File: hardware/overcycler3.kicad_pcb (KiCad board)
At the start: 2 copper layers, 200.7 x 99.1 mm, 309 parts, among them IC1 LM13700, IC2 LM13700, IC3 LM13700, J1 USB_B, J2 AudioJack3_Switch, J3 DIN-5_180degree, J4 AudioJack3_Switch, J5 AudioJack3_Switch, P1 FT232, P2 PANEL, Q1 2SC945, SW1 RESET, SW2 POWER, U1 XT26G02ELGIGA, U10 MCP4922-ESL, U11 SSI2144, U12 MCP4922-ESL, U13 SSI2144, U14 MCP4922-ESL, U15 SSI2144, U16 MCP4922-ESL, U17 SSI2144, U18 MCP4922-ESL, U19 SSI2144, U2 TL074, U20 AD5328B, U3 LPC1778FBD144, U4 TLV1543, U5 74HC138, U6 TL074, U7 AD5328B, U8 MCP4922-ESL, U9 SSI2144, Y1 12MHz

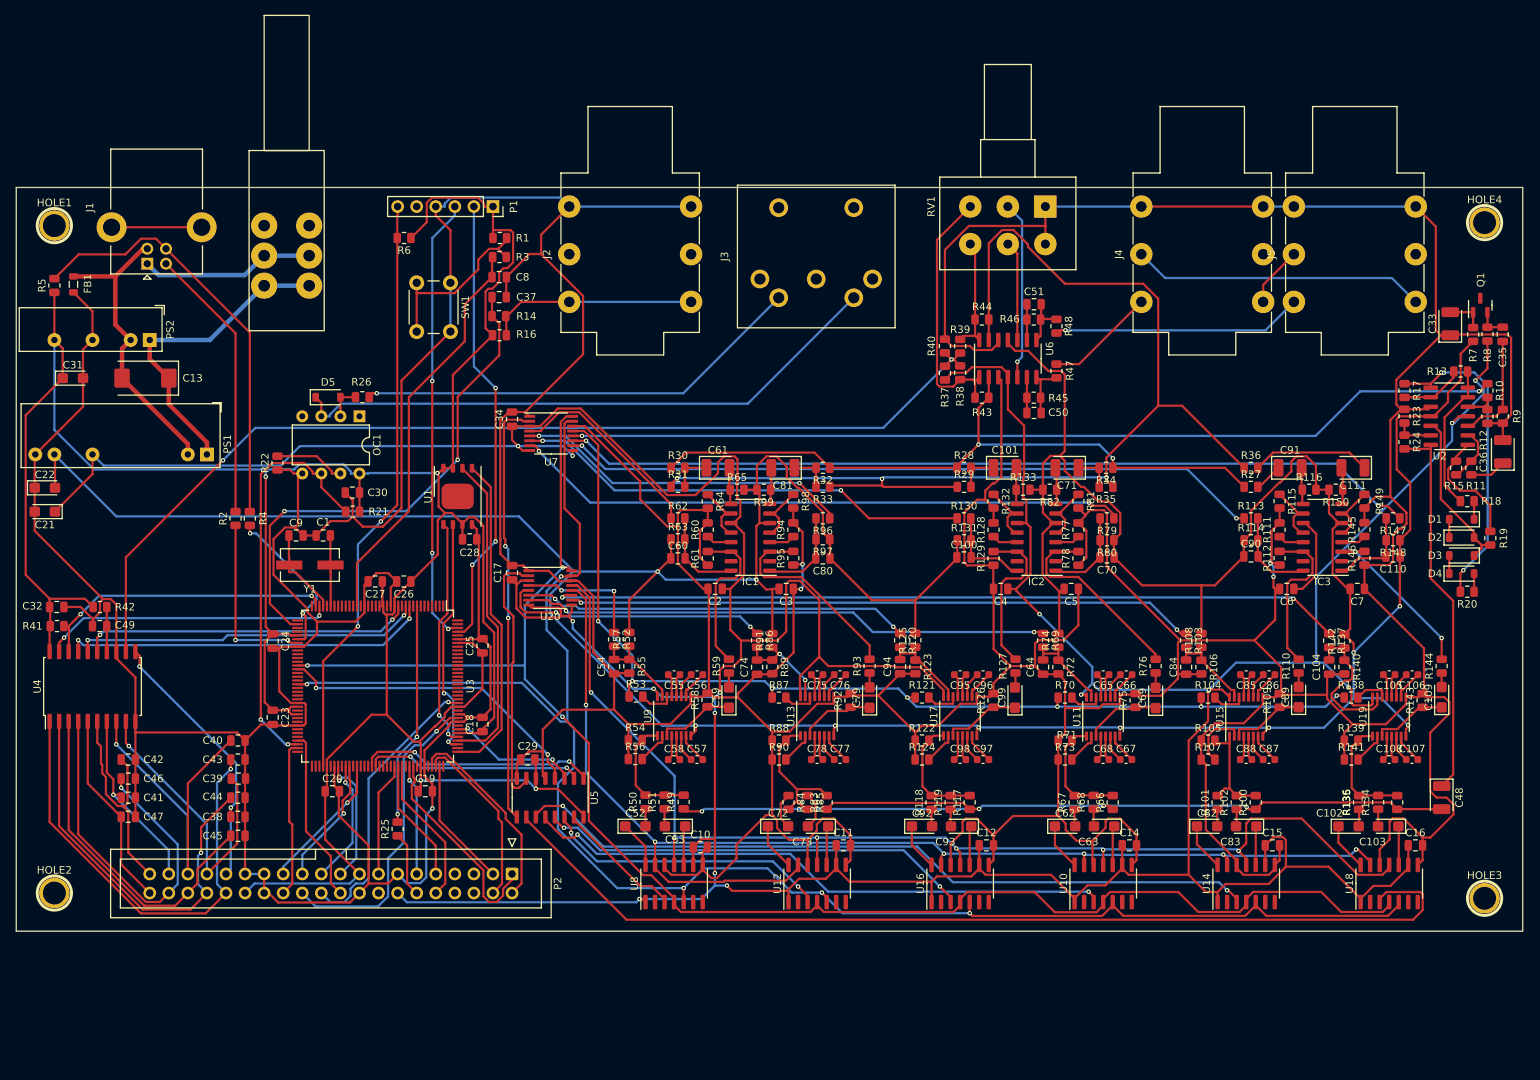
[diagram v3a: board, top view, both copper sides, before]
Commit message: hardware: improved draft routing
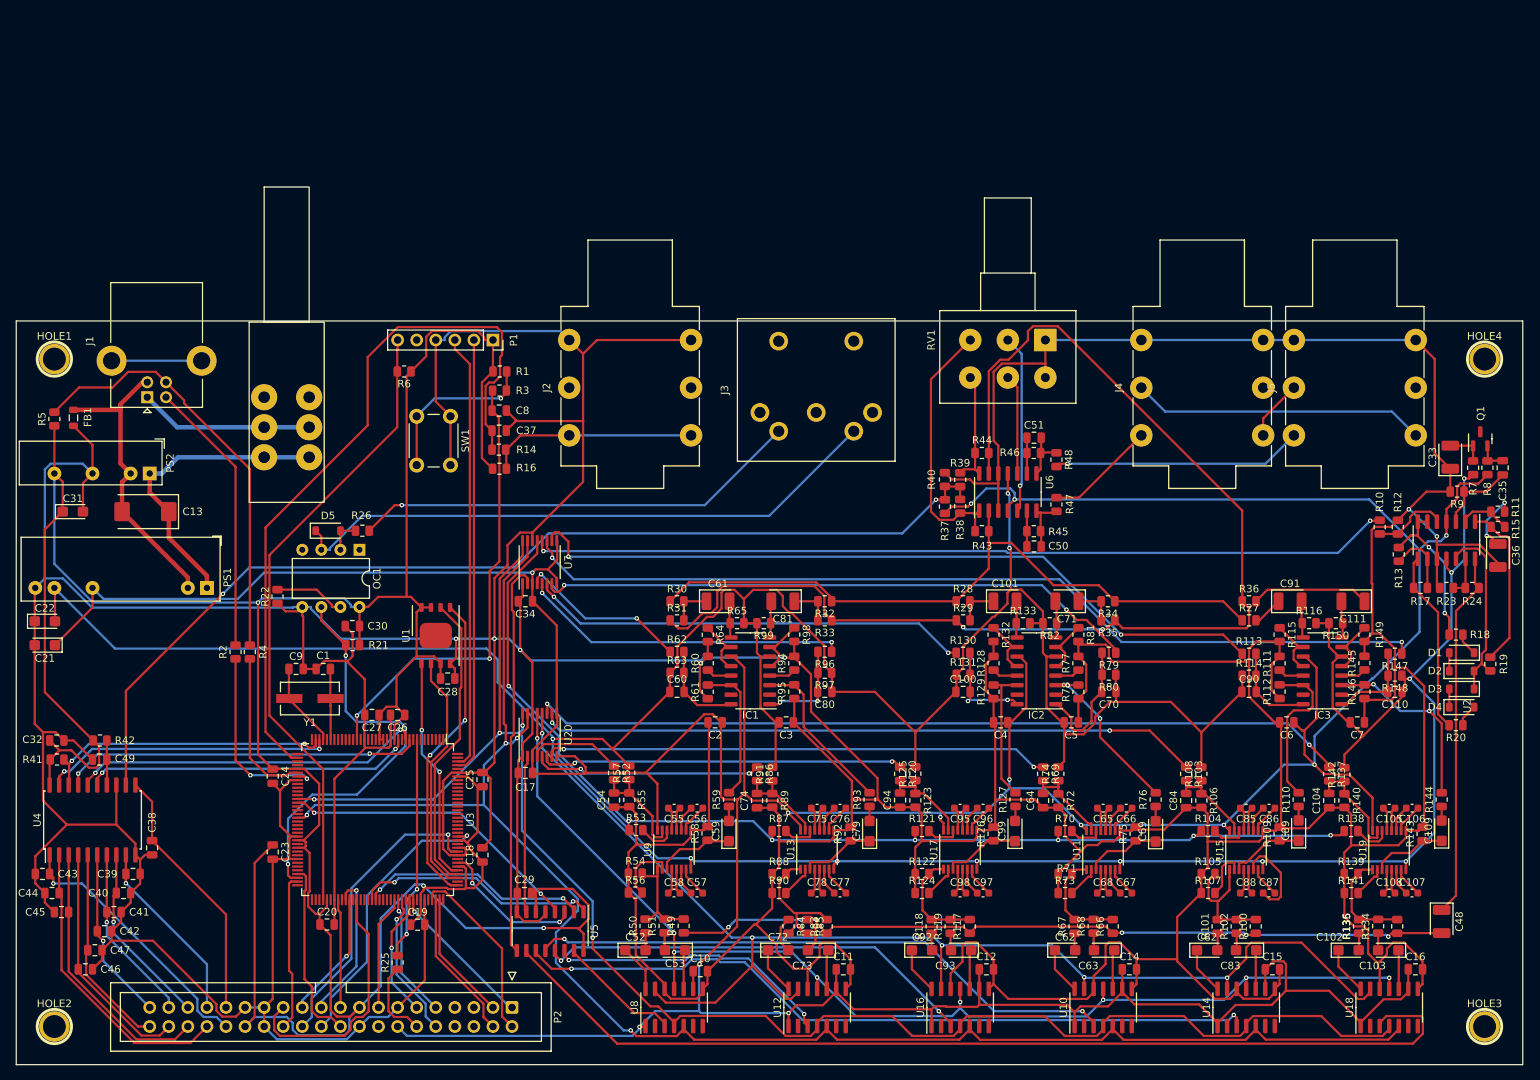
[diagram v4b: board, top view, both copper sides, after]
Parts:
- moved C43 30.2 mm to (23.8, 111.8), turned to 180 degrees
- moved C44 27.8 mm to (25.1, 114.3), turned to 180 degrees
- moved C17 26.7 mm to (88.1, 98.3), turned to 180 degrees
- moved R17 26.4 mm to (207.4, 73.7), turned to 0 degrees
- moved C46 26.0 mm to (29.5, 124.5)
- moved R13 25.7 mm to (204.5, 69.2), turned to -90 degrees
- moved C45 25.6 mm to (26.4, 116.8), turned to 180 degrees
- moved C40 25.4 mm to (34.6, 114.3)
- moved C34 24.3 mm to (88.1, 75.4), turned to 180 degrees
- moved R23 23.6 mm to (210.8, 73.7), turned to 0 degrees
- moved R10 23.2 mm to (201.9, 65.6)
- moved C42 23.1 mm to (32.1, 119.4)
- moved SW2 22.9 mm to (53.3, 48.3)
- moved R24 21.4 mm to (214.2, 73.7), turned to 0 degrees
- moved U20 19.6 mm to (90.0, 93.2), turned to 90 degrees
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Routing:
- net GND: track 1318.7 -> 1351.9 mm, vias 5 -> 7
- net /FOOT_IN: track 68.2 -> 98.3 mm, vias 2 -> 0
- net +3.3V: track 419.5 -> 447.5 mm, vias 4 -> 3
- net /P_0: track 62.1 -> 35.8 mm
- net /P_7: track 44.4 -> 24.6 mm
- net NOISE: track 124.8 -> 105.9 mm, vias 4 -> 5
- net /P_3: track 50.2 -> 31.7 mm, vias 1 -> 0
- net Net-(R17-Pad1): track 42.0 -> 24.3 mm, vias 2 -> 0
- net /KP_4_R4: track 18.4 -> 33.9 mm, vias 1 -> 0
- net /P_8: track 39.5 -> 24.8 mm
- net /P_1: track 54.1 -> 39.8 mm, vias 1 -> 0
- net /SPI_CS7: track 34.8 -> 21.0 mm
- net -5V: track 538.8 -> 527.0 mm, vias 10 -> 12
- net /DAC_MIXN: track 124.7 -> 114.7 mm
- net /P_2: track 45.2 -> 35.9 mm
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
